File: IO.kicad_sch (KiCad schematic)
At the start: 36 parts

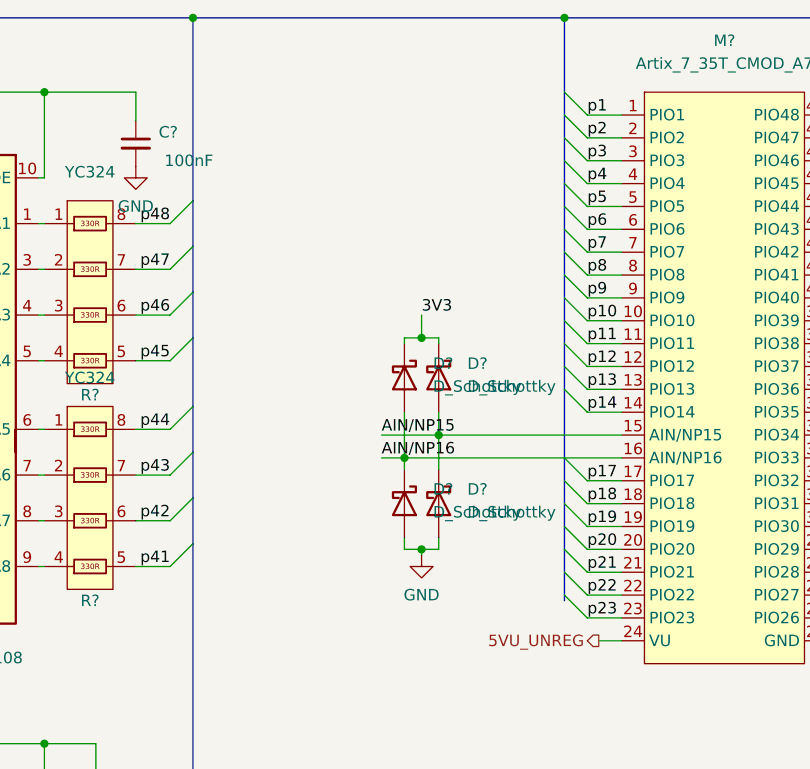
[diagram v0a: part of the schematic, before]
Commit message: Issue #6 fixed
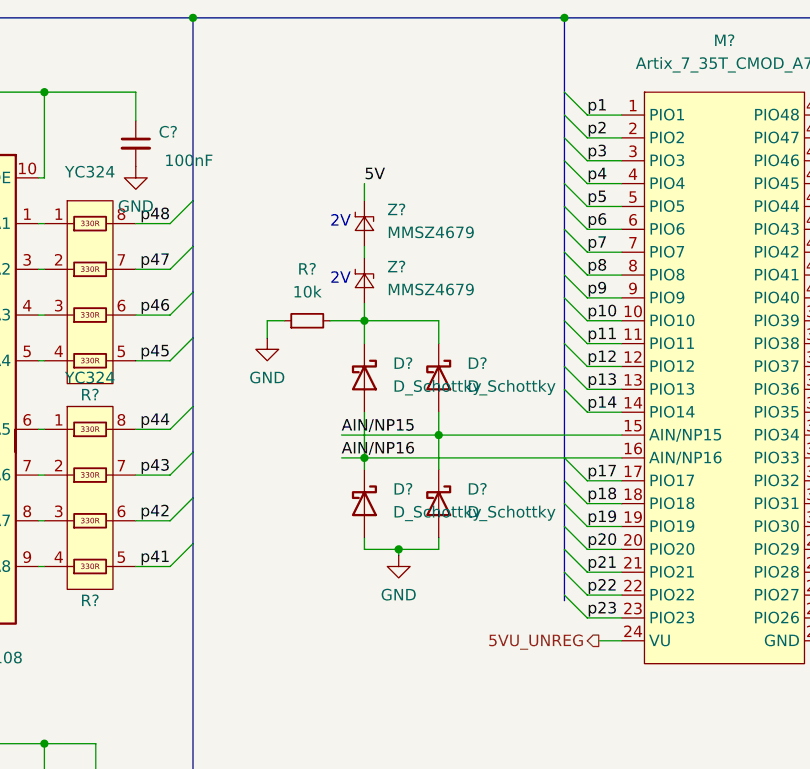
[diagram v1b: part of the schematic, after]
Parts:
- added R?: 10k, symbol Device:R_Small
- added Z? (x2): MMSZ4679, symbol JRIX Diode:MMSZ4679
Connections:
- net 5V: now also Z?.1
- net GND: now also R?.1
- net 3V3: no longer names the net of D?.1 (K), D?.1 (K)
- net 3V3: now also R?.2, Z?.2
- new net: Z?.1, Z?.2
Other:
- note added: "2V"
- moved on the sheet: D?
